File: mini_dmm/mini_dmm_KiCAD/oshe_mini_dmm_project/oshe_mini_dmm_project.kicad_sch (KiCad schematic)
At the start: 11 parts, among them SW1 SW_DPDT_x2, U1 LM358, U2 STM32F303CBTx

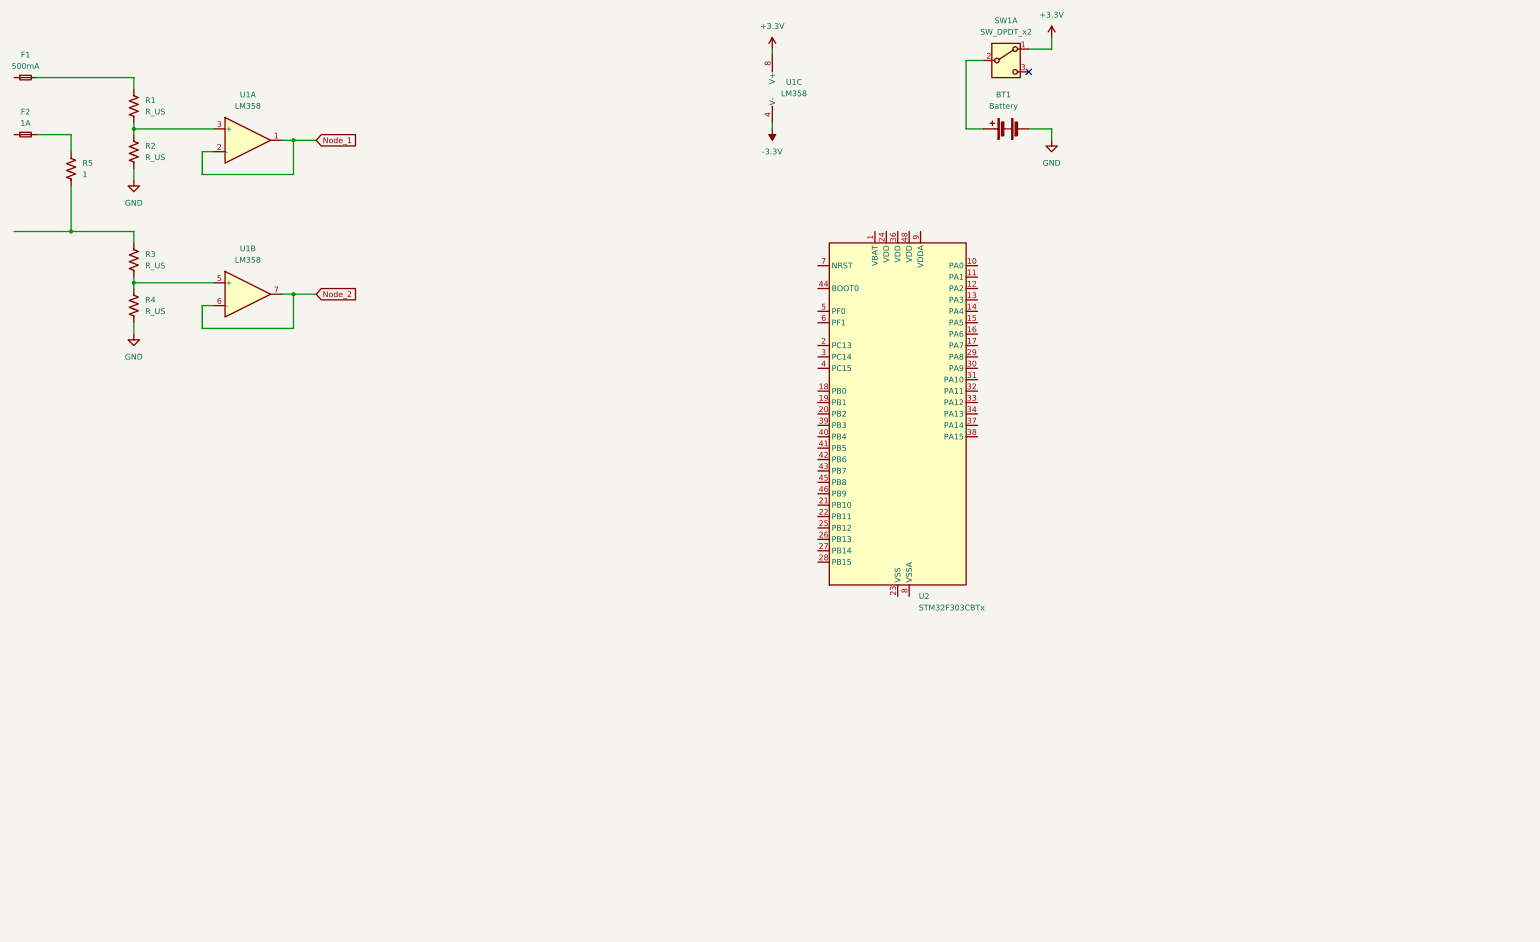
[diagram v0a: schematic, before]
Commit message: Made some more updates!
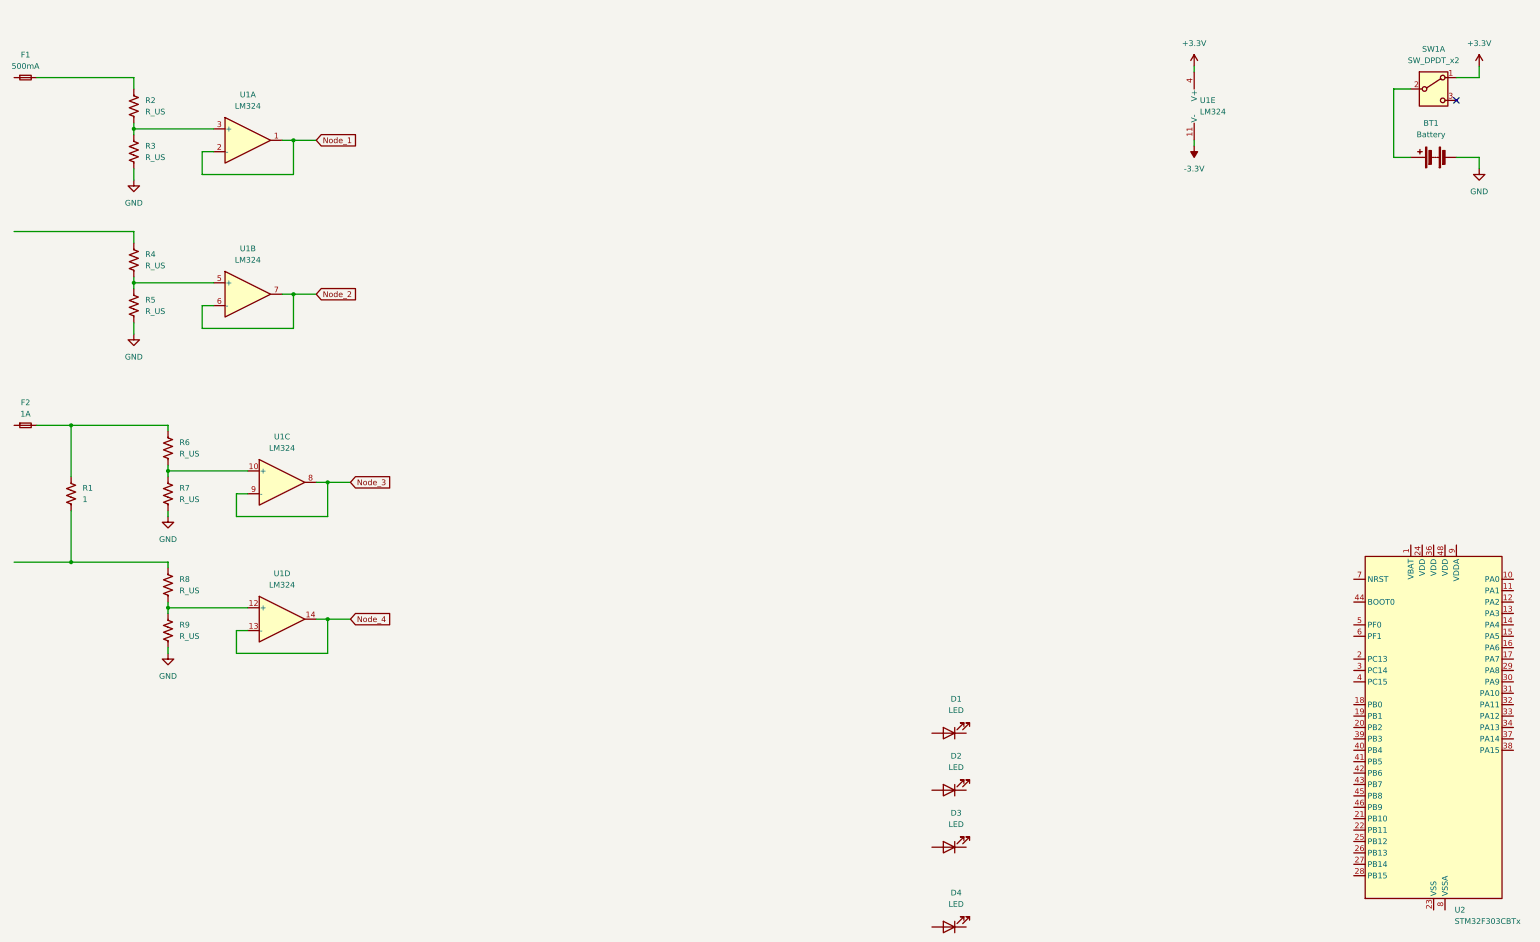
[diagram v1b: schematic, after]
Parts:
- removed U1: LM358, symbol Amplifier_Operational:LM358
- added D1, D2, D3, D4: LED, symbol Device:LED
- added R6, R7, R8, R9: R_US, symbol Device:R_US
- added U1: LM324, Package_SO:SOIC-14_3.9x8.7mm_P1.27mm, symbol Amplifier_Operational:LM324
- renumbered R5 to R1, R1 to R2, R2 to R3, R3 to R4, R4 to R5
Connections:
- net +3.3V: now also U1.4 (V+)
- net -3.3V: now also U1.11 (V-)
- net GND: now also R7.2, R9.2
- net Node_1: now also U1.1, U1.2 (-)
- net Node_2: now also U1.6 (-), U1.7
- net at R2.2, R3.1: now also U1.3 (+)
- net at F2.2, R1.1: now also R6.1
- net at R1.2: now also R8.1; no longer R4.1
- net at R4.2, R5.1: now also U1.5 (+)
- new net: R8.2, R9.1, U1.12 (+)
- new net: R6.2, R7.1, U1.10 (+)
- new net Node_3: U1.8, U1.9 (-)
- new net Node_4: U1.13 (-), U1.14
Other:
- moved on the sheet: BT1, F2, R1, SW1A, U2
